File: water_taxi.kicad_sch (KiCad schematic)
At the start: 17 parts

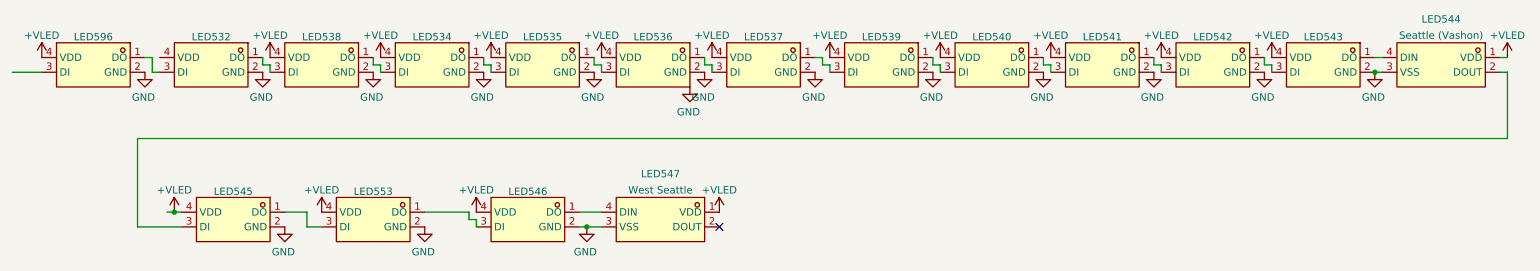
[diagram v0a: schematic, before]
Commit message: checkpoint before label plugin
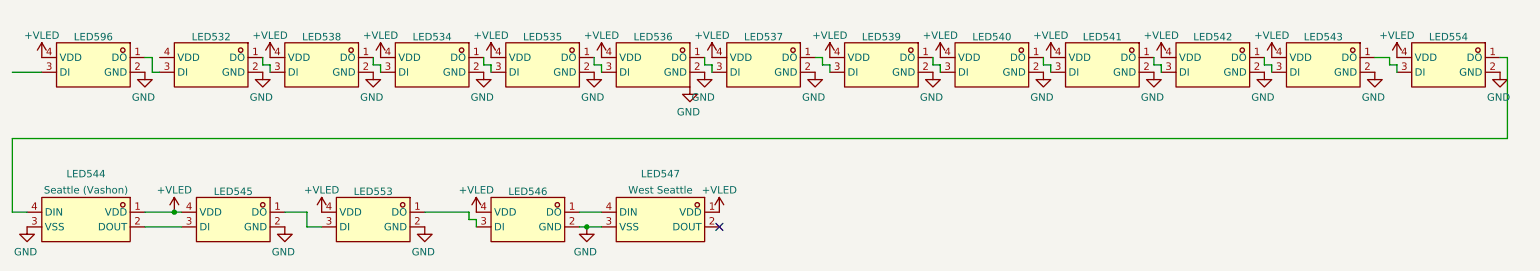
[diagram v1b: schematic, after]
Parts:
- added LED554: WS2812B-2020, EasyEDA:LED-SMD_4P-L2.0-W2.0-TL_WS2812B-2020, symbol EasyEDA:WS2812B-2020
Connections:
- net +VLED: now also LED554.4 (VDD)
- net GND: now also LED554.2 (GND)
- net at LED544.4 (DIN): now also LED554.1 (DO); no longer LED543.1 (DO)
- new net: LED543.1 (DO), LED554.3 (DI)
